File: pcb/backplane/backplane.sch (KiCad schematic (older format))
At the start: 56 parts, among them U1 PCA9685PW, U2 IFX9201SGAUMA1, U3 IFX9201SGAUMA1, U4 IFX9201SGAUMA1, U5 PREC004SAAN-RC, U6 IFX9201SGAUMA1

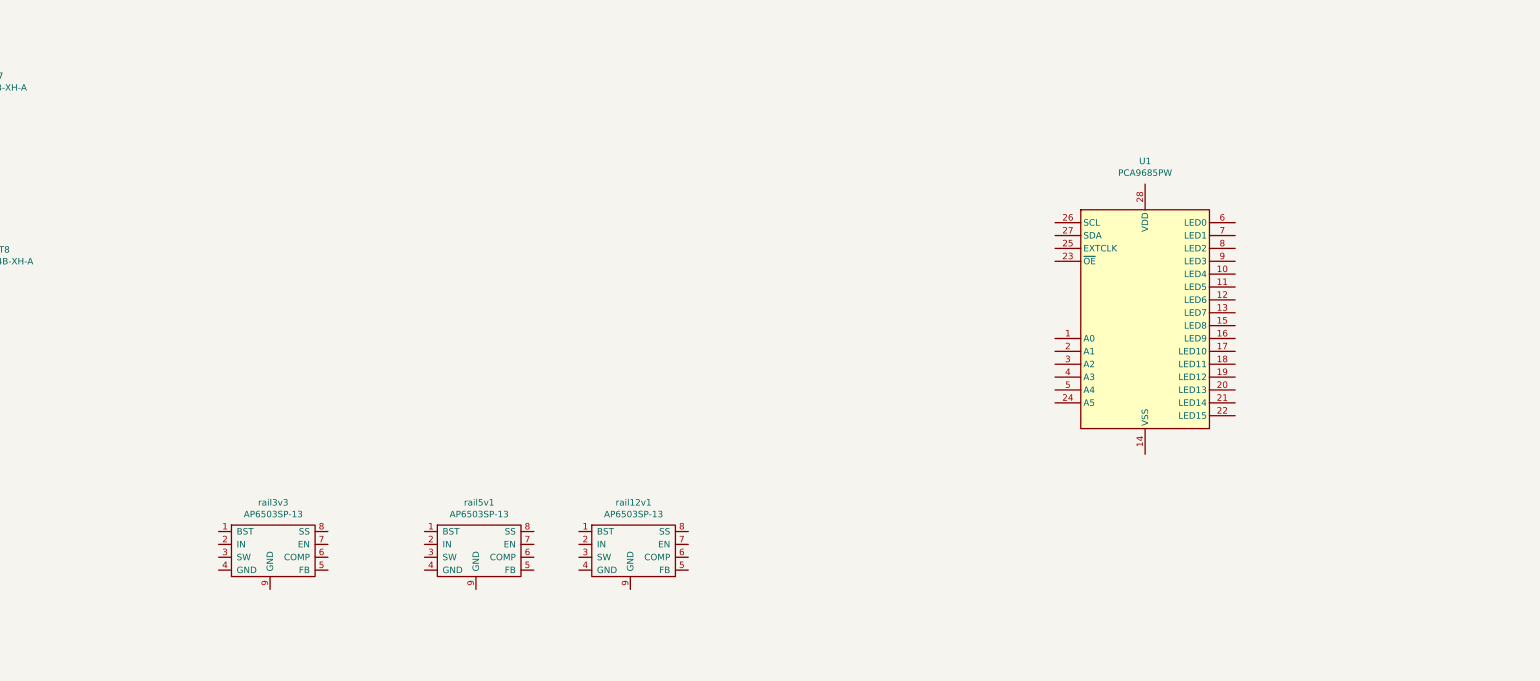
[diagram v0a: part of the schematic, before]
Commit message: updates
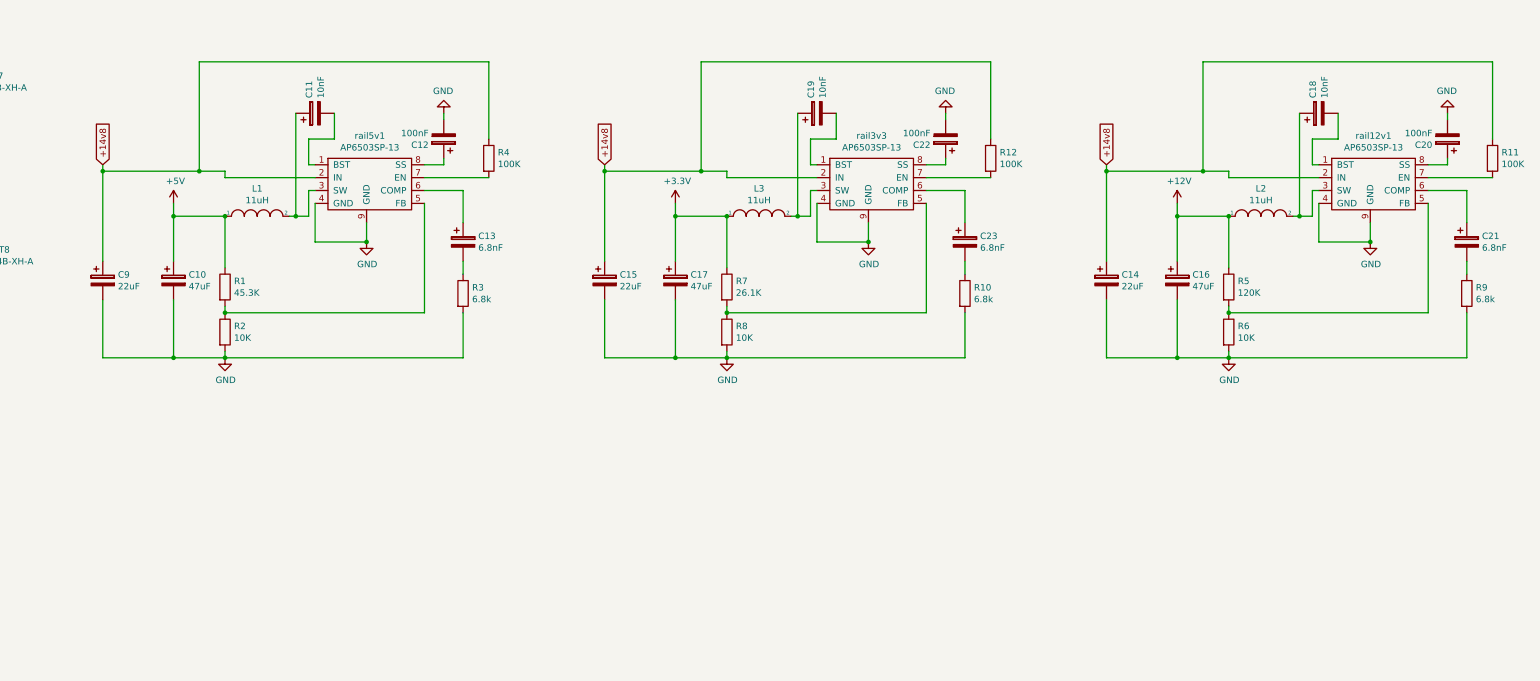
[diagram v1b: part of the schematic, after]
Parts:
- removed U1: PCA9685PW, Package_SO:TSSOP-28_4.4x9.7mm_P0.65mm, symbol Driver_LED:PCA9685PW
- removed rail5v1: AP6503SP-13, backplane:AP6503SP-13, symbol backplane_Library:AP6503SP-13
- added C10, C16, C17: 47uF, backplane:865090449007, symbol Device:CP
- added C11, C18, C19: 10nF, Capacitor_SMD:C_1206_3216Metric_Pad1.42x1.75mm_HandSolder, symbol Device:CP
- added C12, C20, C22: 100nF, Capacitor_SMD:C_1206_3216Metric_Pad1.42x1.75mm_HandSolder, symbol Device:CP
- added C13, C21, C23: 6.8nF, Capacitor_SMD:C_1206_3216Metric_Pad1.42x1.75mm_HandSolder, symbol Device:CP
- added C14, C15, C9: 22uF, backplane:865090442004, symbol Device:CP
- added L1, L2, L3: 11uH, backplane:P0847SNL, symbol pspice:INDUCTOR
- added R1: 45.3K, Resistor_SMD:R_1206_3216Metric_Pad1.42x1.75mm_HandSolder, symbol Device:R
- added R10, R3, R9: 6.8k, Resistor_SMD:R_1206_3216Metric_Pad1.42x1.75mm_HandSolder, symbol Device:R
- added R11, R12, R4: 100K, Resistor_SMD:R_1206_3216Metric_Pad1.42x1.75mm_HandSolder, symbol Device:R
- added R2, R6, R8: 10K, Resistor_SMD:R_1206_3216Metric_Pad1.42x1.75mm_HandSolder, symbol Device:R
- added R5: 120K, Resistor_SMD:R_1206_3216Metric_Pad1.42x1.75mm_HandSolder, symbol Device:R
- added R7: 26.1K, Resistor_SMD:R_1206_3216Metric_Pad1.42x1.75mm_HandSolder, symbol Device:R
- added rail3v3: AP6503SP-13, backplane:AP6503SP-13, symbol backplane_Library:AP6503SP-13
- C5, C6, C7, C8: footprint backplane:865090640001 -> Capacitor_SMD:C_1206_3216Metric_Pad1.42x1.75mm_HandSolder
- renumbered rail3v3 to rail5v1
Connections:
- net +12V: now also C16.1, L2.1, R5.1
- net +14v8: now also rail12v1.2 (IN), rail5v1.2 (IN), C14.1, C15.1, C9.1, R11.1, R12.1, R4.1, rail3v3.2 (IN)
- net +3V3: now also C17.1, L3.1, R7.1
- net +5V: now also C10.1, L1.1, R1.1
- net GND: now also rail12v1.4 (GND), rail12v1.9 (GND), rail5v1.4 (GND), rail5v1.9 (GND), C10.2, C12.2, C14.2, C15.2, C16.2, C17.2, C20.2, C22.2, C9.2, R10.2, R2.2, R3.2, R6.2, R8.2, R9.2, rail3v3.4 (GND), rail3v3.9 (GND)
- net at rail5v1.1 (BST): now also C11.2
- net at rail5v1.3 (SW): now also C11.1, L1.2
- net at rail5v1.5 (FB): now also R1.2, R2.1
- net at rail5v1.6 (COMP): now also C13.1
- net at rail5v1.7 (EN): now also R4.2
- net at rail5v1.8 (SS): now also C12.1
- net at rail12v1.1 (BST): now also C18.2
- net at rail12v1.3 (SW): now also C18.1, L2.2
- net at rail12v1.5 (FB): now also R5.2, R6.1
- net at rail12v1.6 (COMP): now also C21.1
- net at rail12v1.7 (EN): now also R11.2
- net at rail12v1.8 (SS): now also C20.1
- new net: C13.2, R3.1
- new net: C19.2, rail3v3.1 (BST)
- new net: C19.1, L3.2, rail3v3.3 (SW)
- new net: R7.2, R8.1, rail3v3.5 (FB)
- new net: C23.1, rail3v3.6 (COMP)
- new net: R12.2, rail3v3.7 (EN)
- new net: C22.1, rail3v3.8 (SS)
- new net: C23.2, R10.1
- new net: C21.2, R9.1
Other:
- moved on the sheet: rail5v1
